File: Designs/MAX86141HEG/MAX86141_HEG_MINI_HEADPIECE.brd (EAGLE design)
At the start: 252.5 x 37.7 mm, 10 parts, among them U1 OS103012MU2QP1

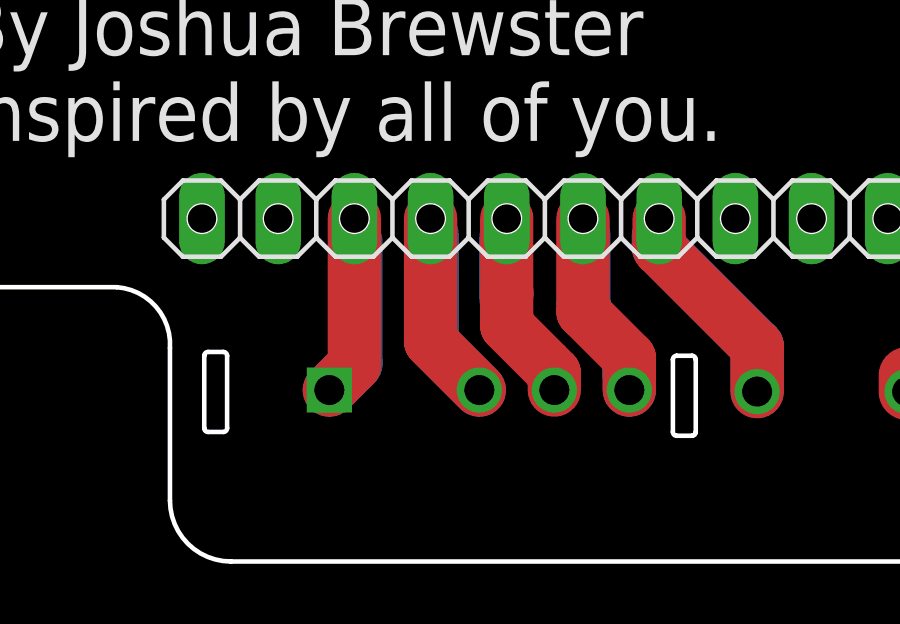
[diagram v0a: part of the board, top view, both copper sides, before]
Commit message: pushed firmware updates
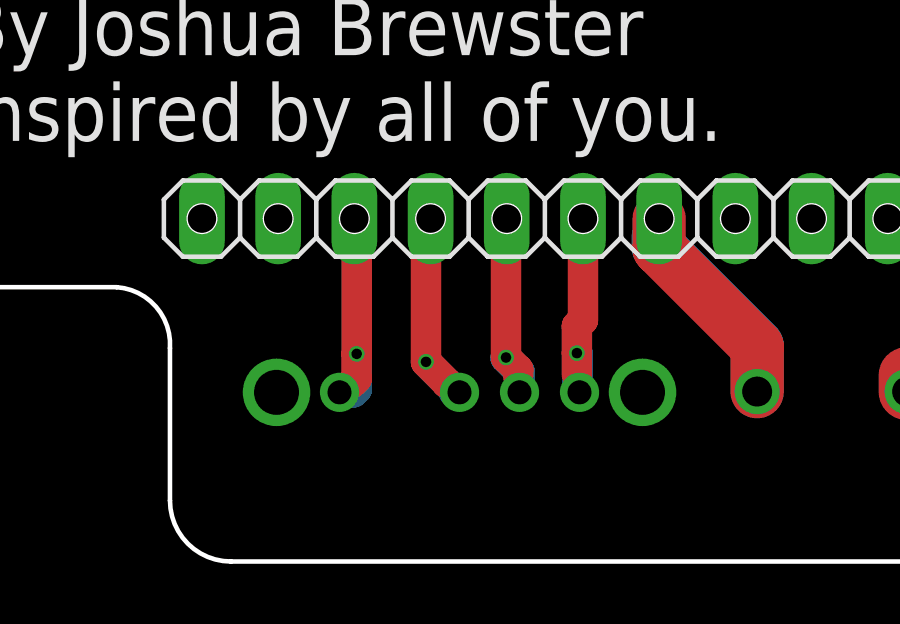
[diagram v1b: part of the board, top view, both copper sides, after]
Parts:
- removed U1: OS103012MU2QP1, OS103012MU2QP1:SW_OS103012MU2QP1
- added S2: OS103011MS8QP1, OS103011MS8QP1:OS102011MS8QP1
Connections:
- removed net N$1: JP1.3, U1.1
- removed net N$2: JP1.4, U1.2
- removed net N$3: JP1.5, U1.3
- removed net N$4: JP1.6, U1.4
- new net 12: JP1.4, S2.2
- new net 13: JP1.3, S2.1
- new net 14: JP1.5, S2.3
- new net 27: JP1.6, S2.4
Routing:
- net N$3: track 15.0 -> 0.00 mm
- net N$2: track 12.2 -> 0.00 mm
- net N$4: track 12.2 -> 0.00 mm
- net N$1: track 11.4 -> 0.00 mm
- net 12: track 0.00 -> 7.42 mm, vias 0 -> 1
- net 13: track 0.00 -> 7.38 mm, vias 0 -> 1
- net 14: track 0.00 -> 6.79 mm, vias 0 -> 1
- net 27: track 0.00 -> 6.64 mm, vias 0 -> 1
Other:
- outline, holes or cut-outs redrawn
